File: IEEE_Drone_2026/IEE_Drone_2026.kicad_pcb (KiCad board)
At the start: 4 copper layers, 49.1 x 55 mm, 48 parts, among them IC1 TPSM84209RKHT, J1 ESC, J10 M2, J12 RF, J13 USB_C_Receptacle_USB2.0_16P, J2 M4 Mounting, J3 M4 Mounting, J4 M4 Mounting, J5 M4 Mounting, J6 Pixy2, J7 M2, J8 M2, J9 M2, U2 STM32F405RGTx, U3 BMP390, U5 LIS2MDL, Y2 ABMM2-32.768MHZ-E2F-T

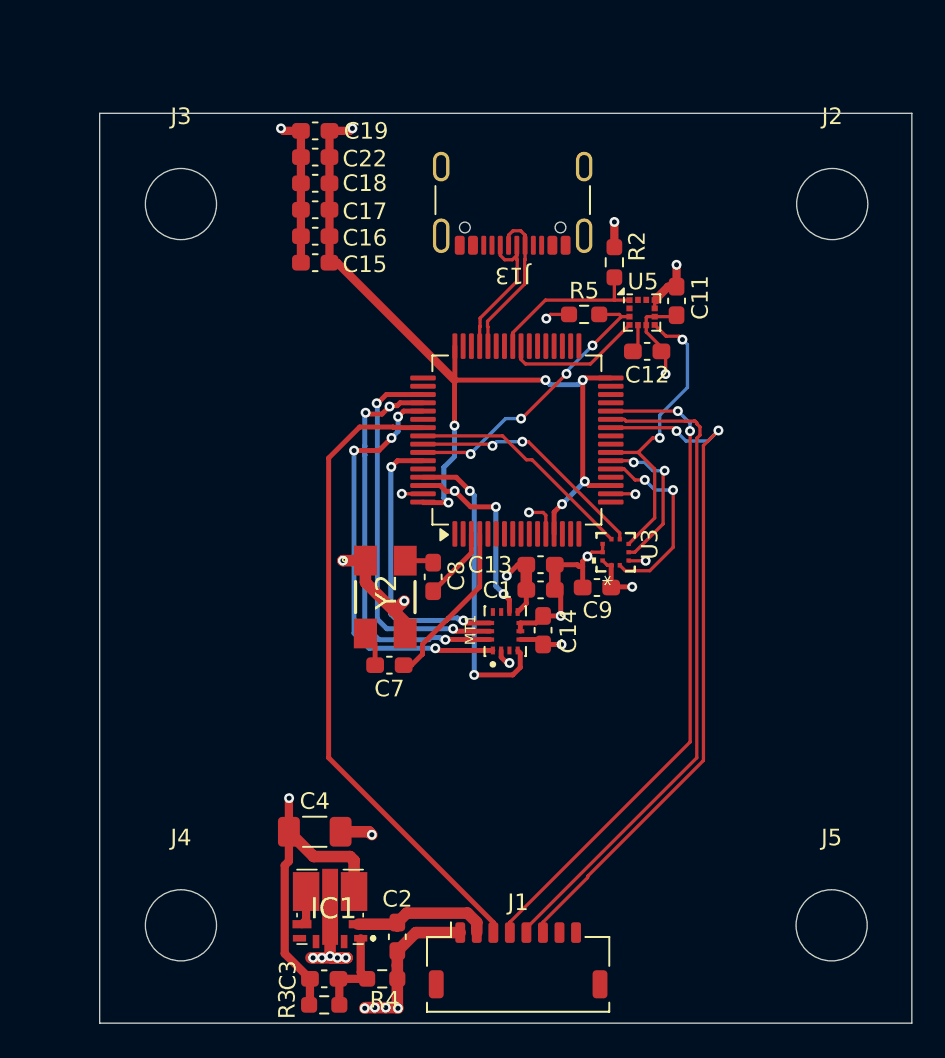
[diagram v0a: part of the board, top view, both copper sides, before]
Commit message: completely updated design
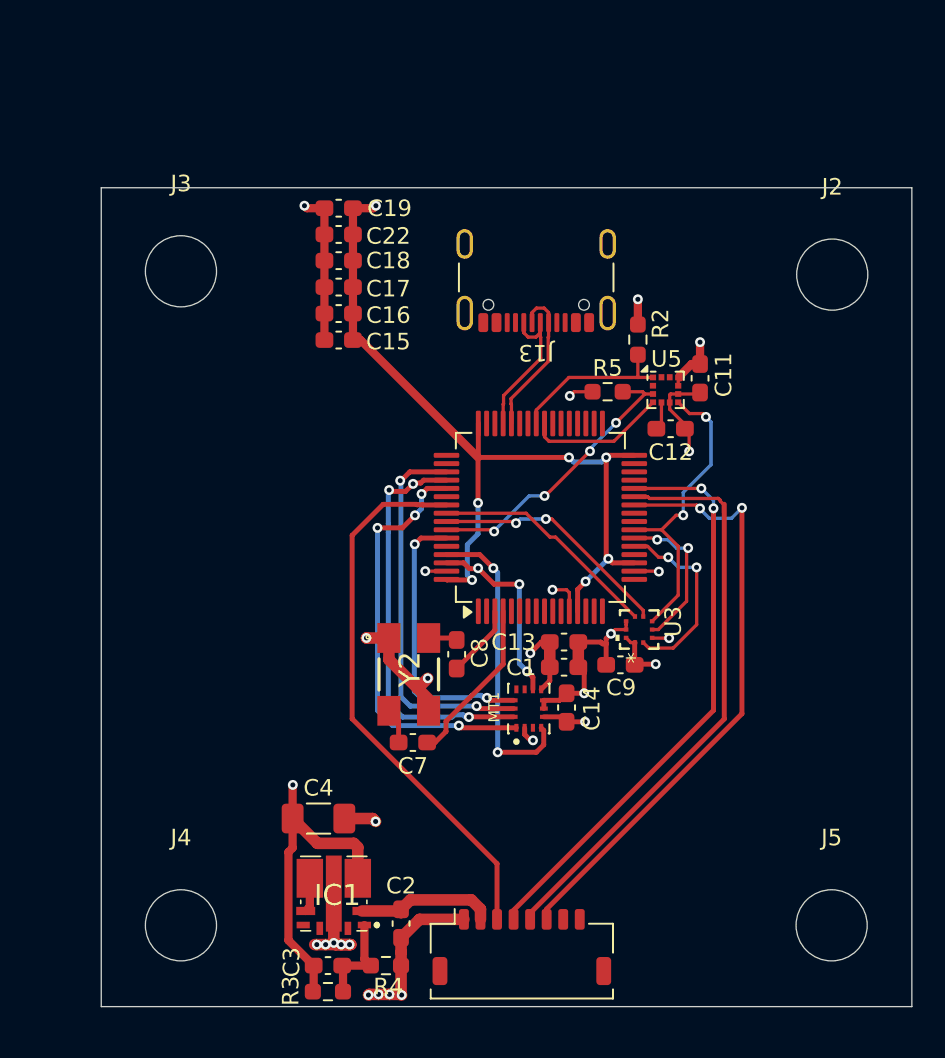
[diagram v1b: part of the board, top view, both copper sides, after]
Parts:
- moved R2 4.89 mm to (95.4, 90.7)
- moved C1 4.89 mm to (91.0, 110.5)
- moved C14 4.89 mm to (91.1, 112.9)
- moved C18 4.89 mm to (77.4, 85.9)
- moved C8 4.89 mm to (84.5, 109.7)
- moved U5 4.89 mm to (97.1, 93.7)
- moved Y2 4.89 mm to (81.6, 110.9)
- moved C12 4.89 mm to (97.4, 96.1)
- moved C9 4.89 mm to (94.4, 110.3)
- moved J13 4.89 mm to (89.3, 86.0)
- moved R5 4.89 mm to (93.6, 93.8)
- moved U3 4.89 mm to (95.5, 108.2)
- moved C11 4.89 mm to (99.2, 93.0)
- moved C13 4.89 mm to (91.0, 109.0)
- moved C15 4.89 mm to (77.4, 90.7)
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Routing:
- net /PB0: track 41.9 -> 36.9 mm
- net /PB2: track 40.5 -> 35.5 mm
- net /PB1: track 41.0 -> 36.1 mm
- net /PB3: track 39.9 -> 44.4 mm
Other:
- board size 49.1 x 55 mm -> 49 x 49.5 mm
